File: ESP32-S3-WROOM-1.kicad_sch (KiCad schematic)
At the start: 24 parts, among them J11 Conn_01x08, J13 Conn_02x09_Top_Bottom, J14 Conn_01x09, J15 Conn_02x09_Top_Bottom, J4 B4B-ZRLFSN, J6 Conn_01x09, J7 Conn_02x20_Counter_Clockwise, J8 Conn_01x08, J9 Conn_01x08, SW4 SW_Push, U8 ESP32-S3-WROOM-1-N8R2

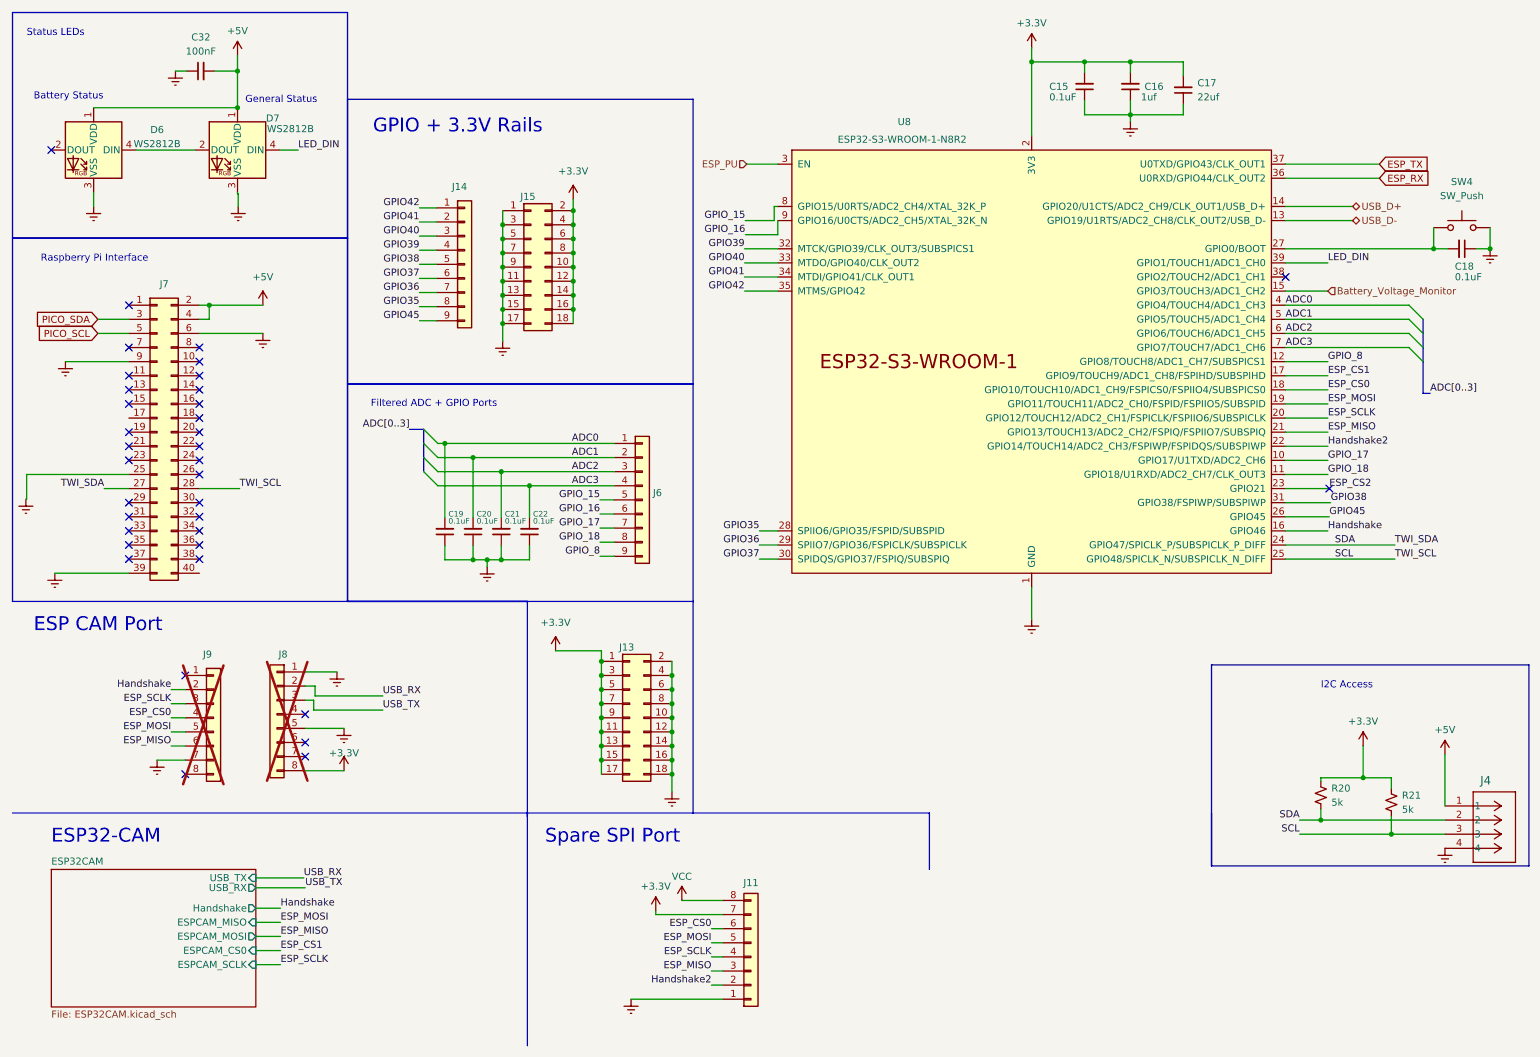
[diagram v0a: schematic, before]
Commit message: clean up Rev
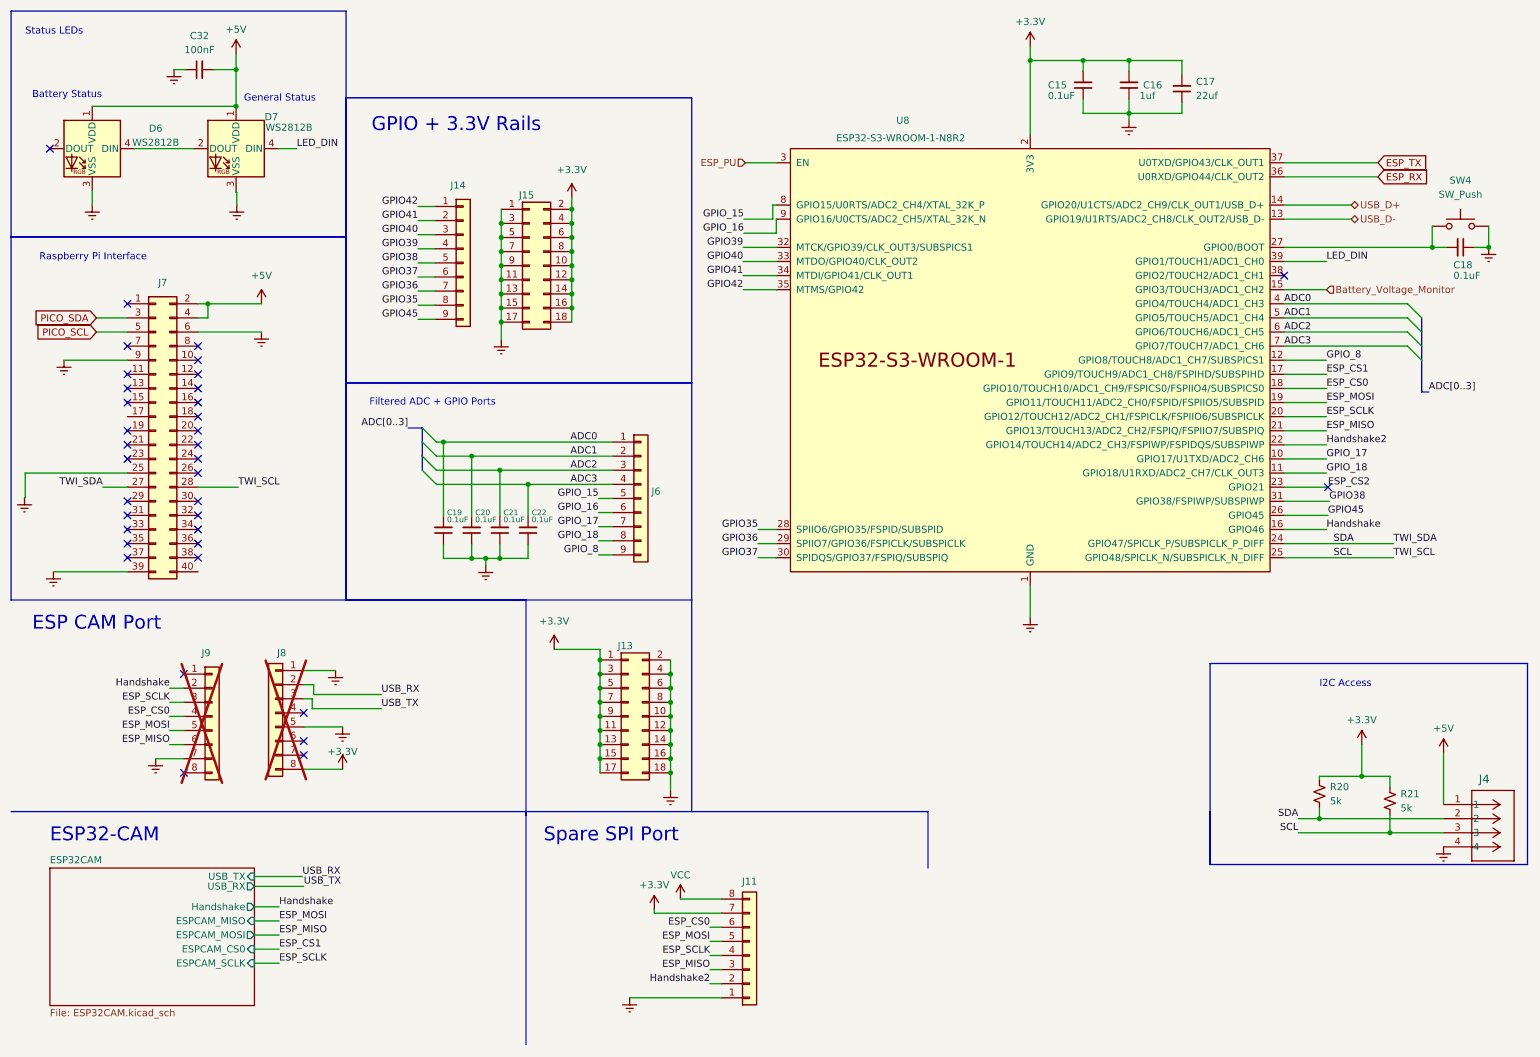
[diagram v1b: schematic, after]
